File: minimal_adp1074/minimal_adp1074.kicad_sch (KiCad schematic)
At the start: 71 parts, among them Q1 80 V, Q2 -60 V, Q3 40 V, Q4 40 V, Q5 150 V, T1 PL160X9-102L-BLD, U1 ADP1074ACCZ-R7

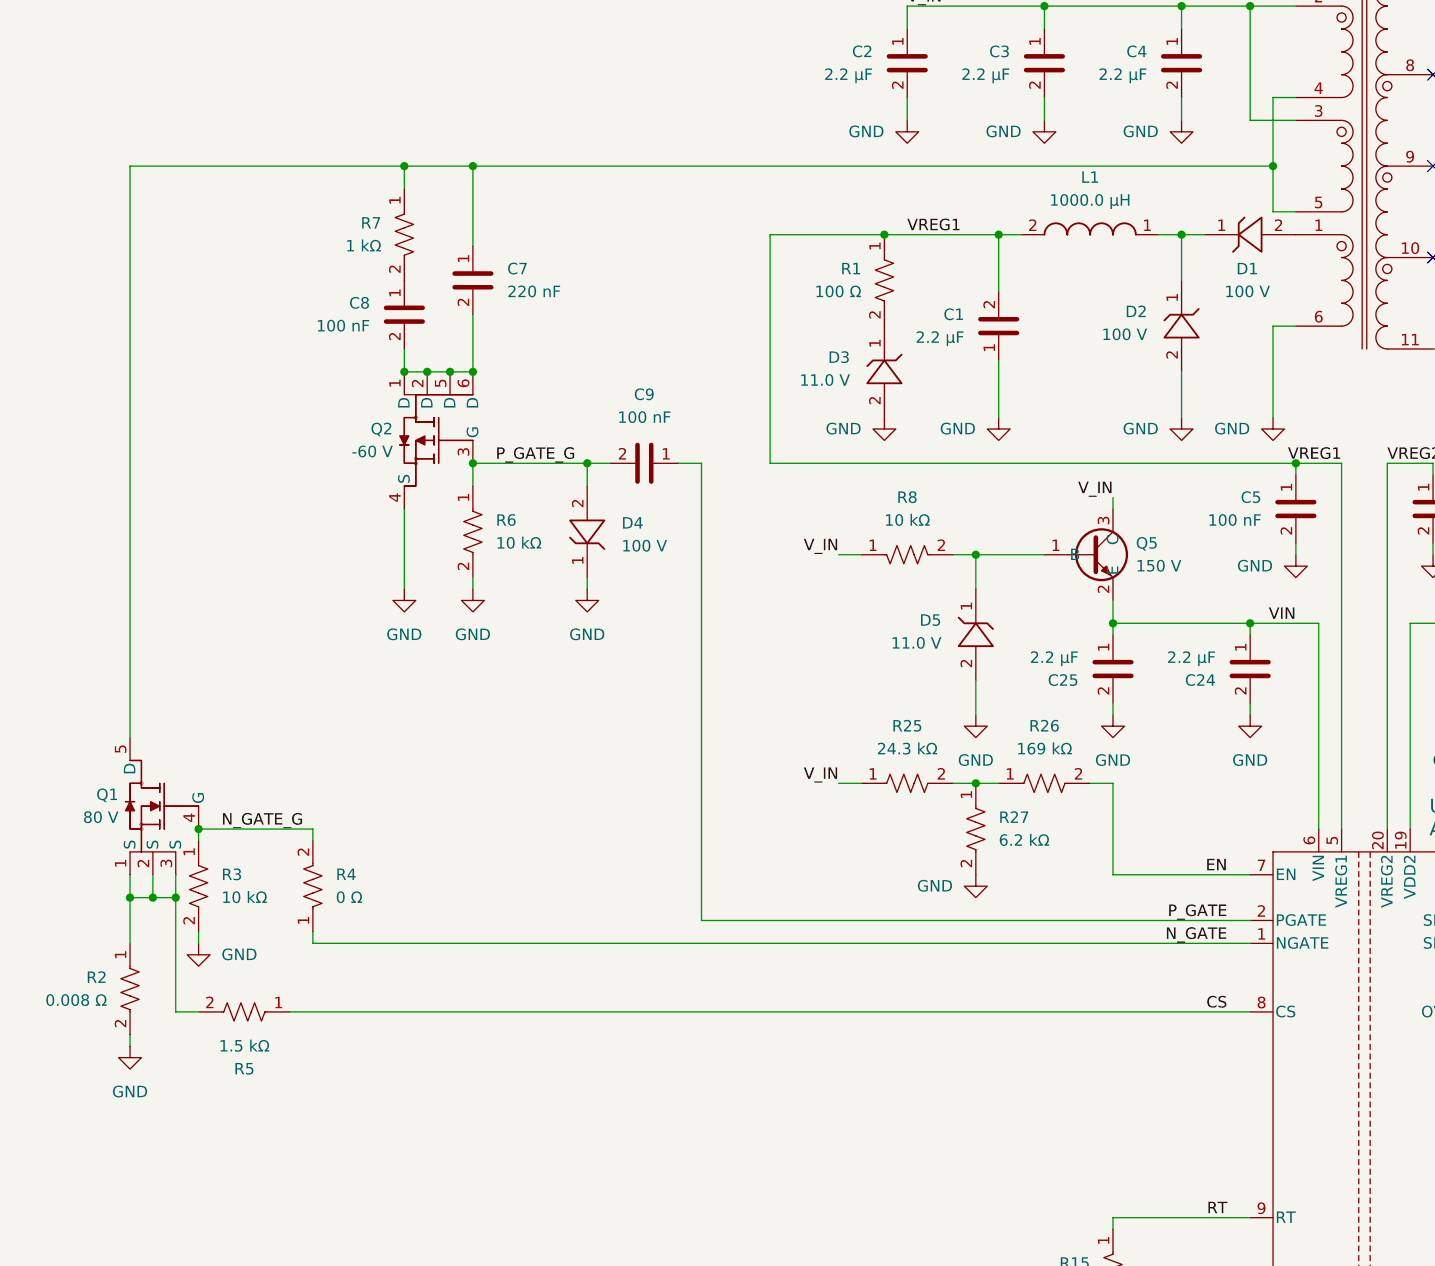
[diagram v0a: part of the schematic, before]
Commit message: backup
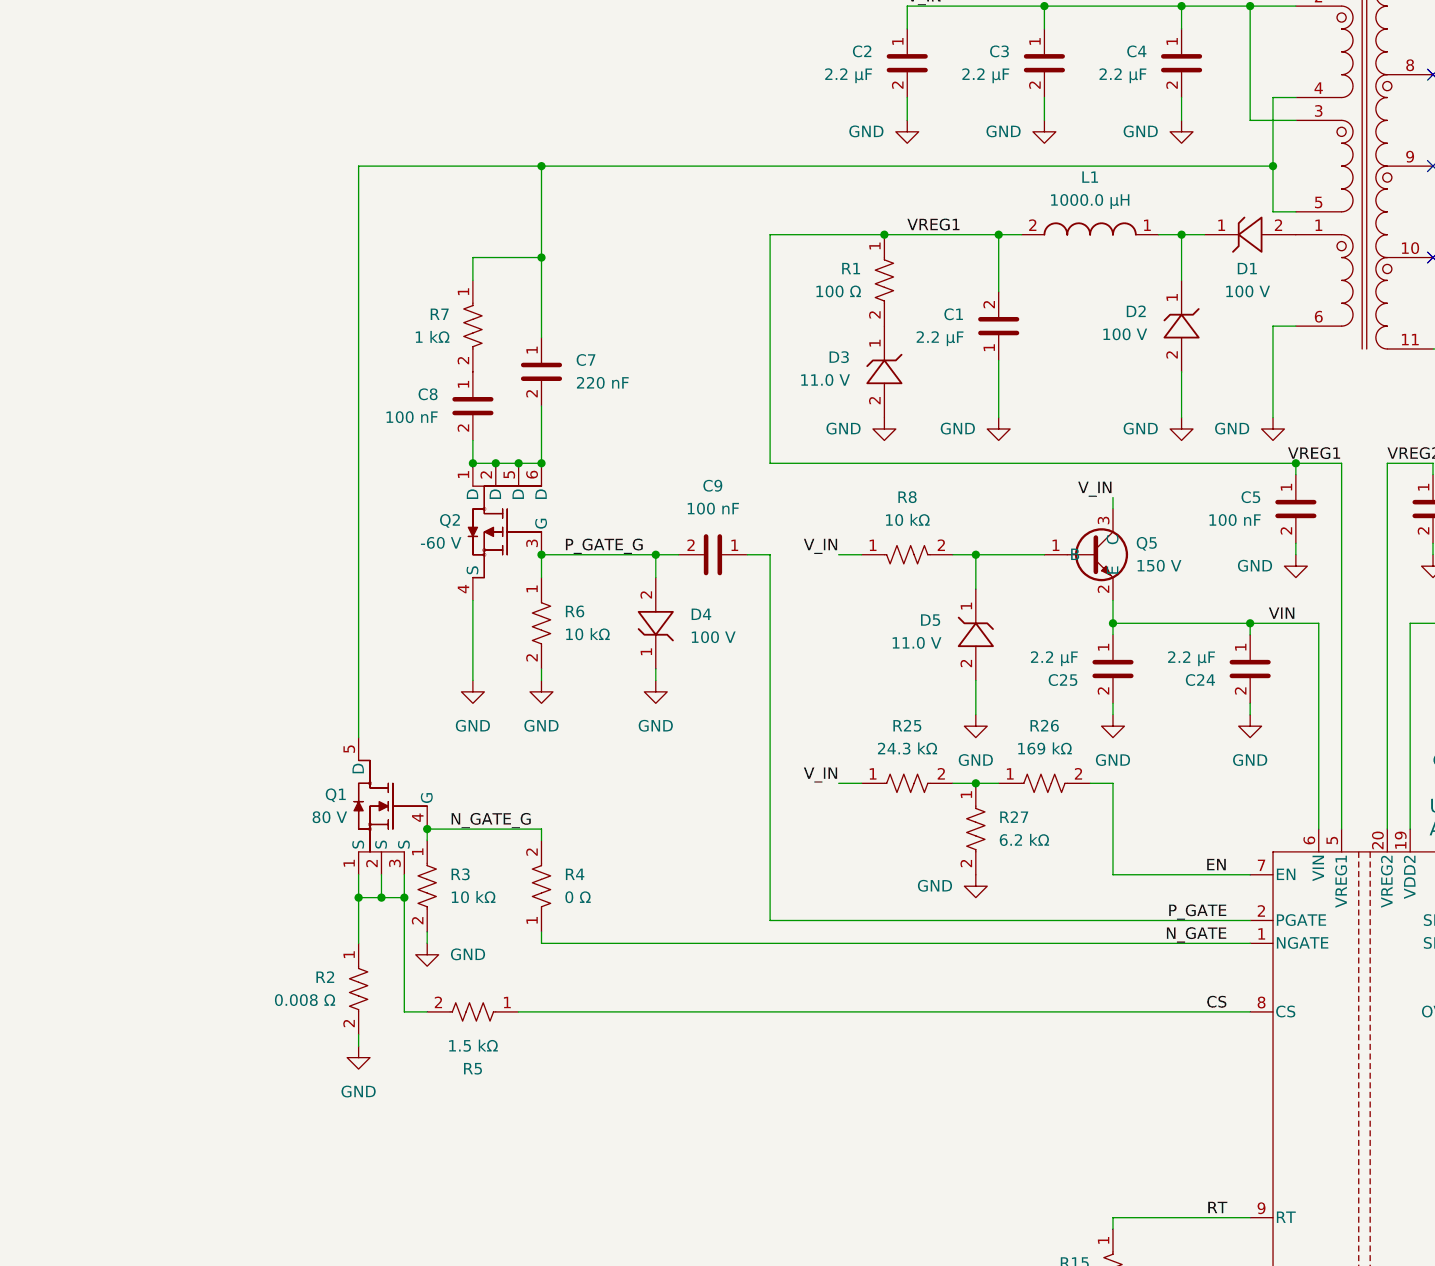
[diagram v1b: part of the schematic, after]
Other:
- moved on the sheet: C7, C8, C9, D4, Q1, Q2, R2, R3, R4, R5, R6, R7
